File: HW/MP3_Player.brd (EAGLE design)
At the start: 160 x 20 mm, 76 parts, among them J1 ISP/SPI, J2 LIPO-BATTERY-CONNECTOR, J3 USD-SDIO-SOCKETJLH, Q2 12.288MHz, U1 3.3V/150mA, U2 1.8V/100mA, U3 ATMEGA32U2, U4 VS1053B, U5 MCP73831

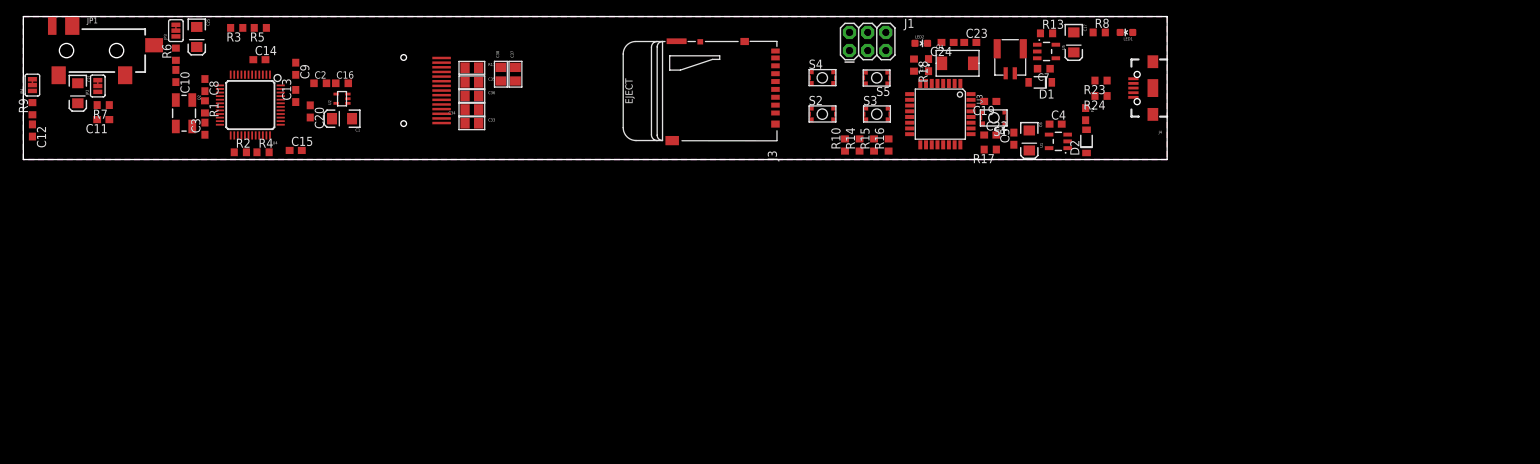
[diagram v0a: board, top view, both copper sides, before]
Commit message: added 3d model. new button.
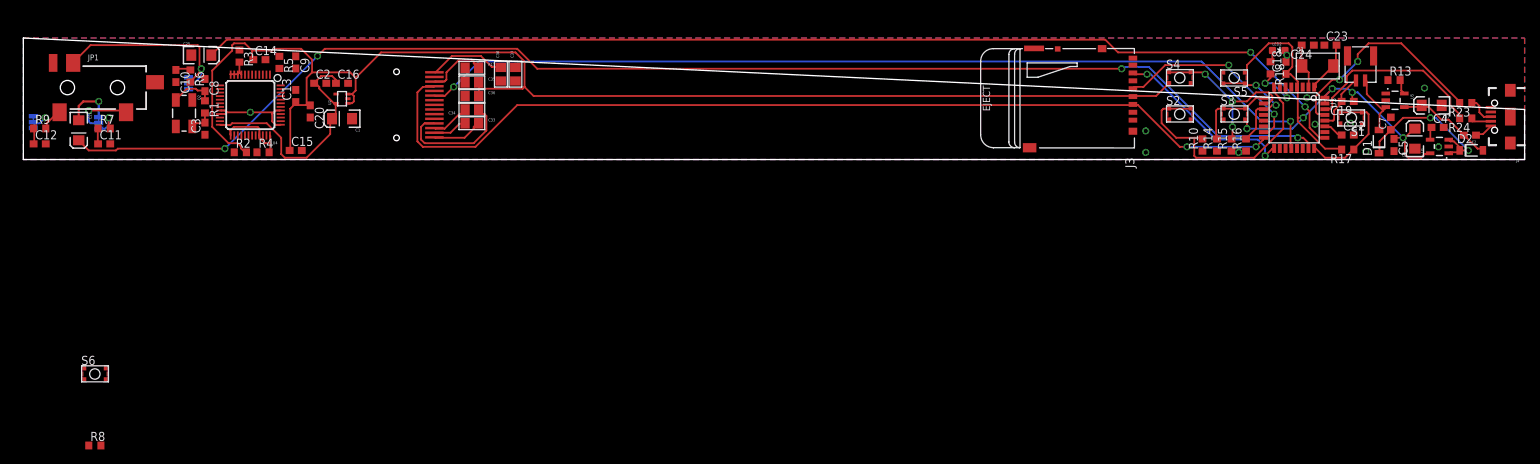
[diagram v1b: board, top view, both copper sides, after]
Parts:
- removed J1: ISP/SPI, SparkFun:2X3
- removed LED1: RED, SparkFun-LED:LED-0603
- added S6: Vol Down, pero_library:TACTILE-SWITCH-SKSGAAE010
- C16, C2: device rcl:C0603K -> rcl:C0603
- C18: device SparkFun-Capacitors:0603-CAP -> rcl:C0603
- R8: value 330 -> 10k
- S5: value Reserved -> Vol Up
- moved R8 151.9 mm to (10.0, -40.0)
- moved C6 53.9 mm to (194.7, 2.92), turned to 90 degrees
- moved F2 53.8 mm to (202.3, 3.41), turned to 180 degrees
- moved D2 53.8 mm to (202.5, 1.28), turned to 0 degrees
- moved C4 53.4 mm to (197.8, 4.49)
- moved U1 53.3 mm to (198.1, 1.83)
- moved C5 53.2 mm to (191.7, 2.03), turned to 270 degrees
- moved R23 51.1 mm to (201.8, 7.92)
- moved R24 51.1 mm to (201.8, 5.76)
- moved C17 50.8 mm to (197.0, 7.57), turned to 180 degrees
- moved C23 50.4 mm to (182.8, 16.0)
- moved C24 50.4 mm to (179.7, 16.0)
- moved Q1 50.4 mm to (181.1, 13.1)
- moved J4 50.2 mm to (208.0, 6.00)
- moved LED2 50.0 mm to (175.6, 15.3)
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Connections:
- removed net 5V-MOSI: J1.4
- removed net 5V-SCK: J1.3
- net 3.3V: now also S6.P$2, S6.P$4; no longer R8.2
- net GND: now also R8.1; no longer J1.6, LED1.C
- net MISO: no longer J1.1
- net N$1: now also U3.21; no longer U3.12
- net N$6: now also R8.2, S6.P$1, S6.P$3, U3.12; no longer LED1.A, R8.1
- net VCC: no longer J1.2
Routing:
- net 3.3V: track 0.00 -> 260.7 mm, vias 0 -> 5
- net PWM_L: track 0.00 -> 185.0 mm, vias 0 -> 4
- net PWM_R: track 0.00 -> 163.7 mm, vias 0 -> 2
- net MOSI: track 0.00 -> 133.8 mm, vias 0 -> 2
- net OLED-DC: track 0.00 -> 129.0 mm, vias 0 -> 2
- net N$18: track 0.00 -> 35.9 mm
- net 1.8V: track 0.00 -> 33.7 mm
- net N$22: track 0.00 -> 30.9 mm, vias 0 -> 2
- net RIGHT: track 0.00 -> 28.5 mm, vias 0 -> 1
- net SCK: track 0.00 -> 27.9 mm, vias 0 -> 2
- net N$23: track 0.00 -> 26.1 mm
- net MISO: track 0.00 -> 25.7 mm, vias 0 -> 2
- net N$27: track 0.00 -> 24.3 mm, vias 0 -> 3
- net VIN: track 0.00 -> 22.9 mm, vias 0 -> 2
- net GND: track 0.00 -> 21.5 mm, vias 0 -> 11
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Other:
- board size 160 x 20 mm -> 210 x 17 mm
